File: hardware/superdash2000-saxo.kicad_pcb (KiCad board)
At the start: 2 copper layers, 77.5 x 59.7 mm, 21 parts, among them IC1 MAX4617CPE+, J1 Molex 34691-0161, U1 L7805, U2 TLV2372

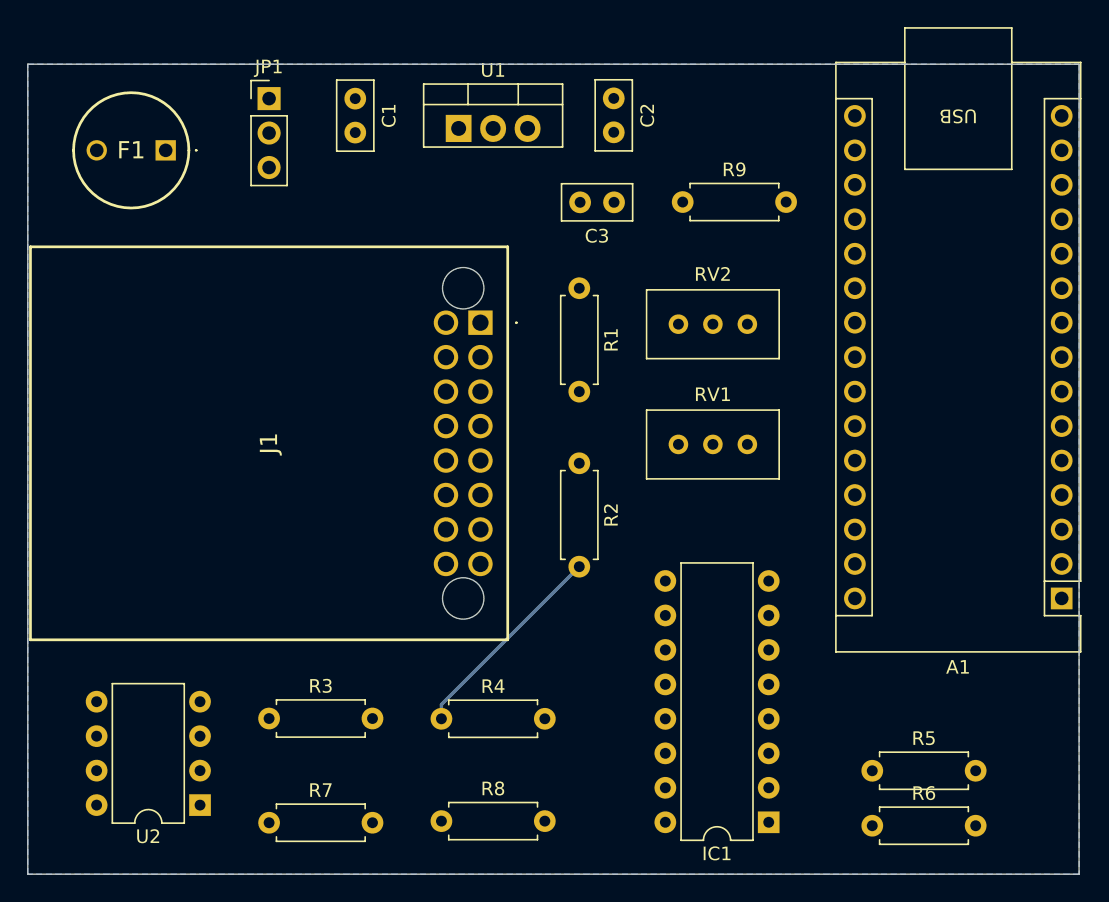
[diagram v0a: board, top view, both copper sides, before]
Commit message: hardware: Update pcb
Signed-off-by: Thomas Antonini <antonini.thomas@gmail.com>
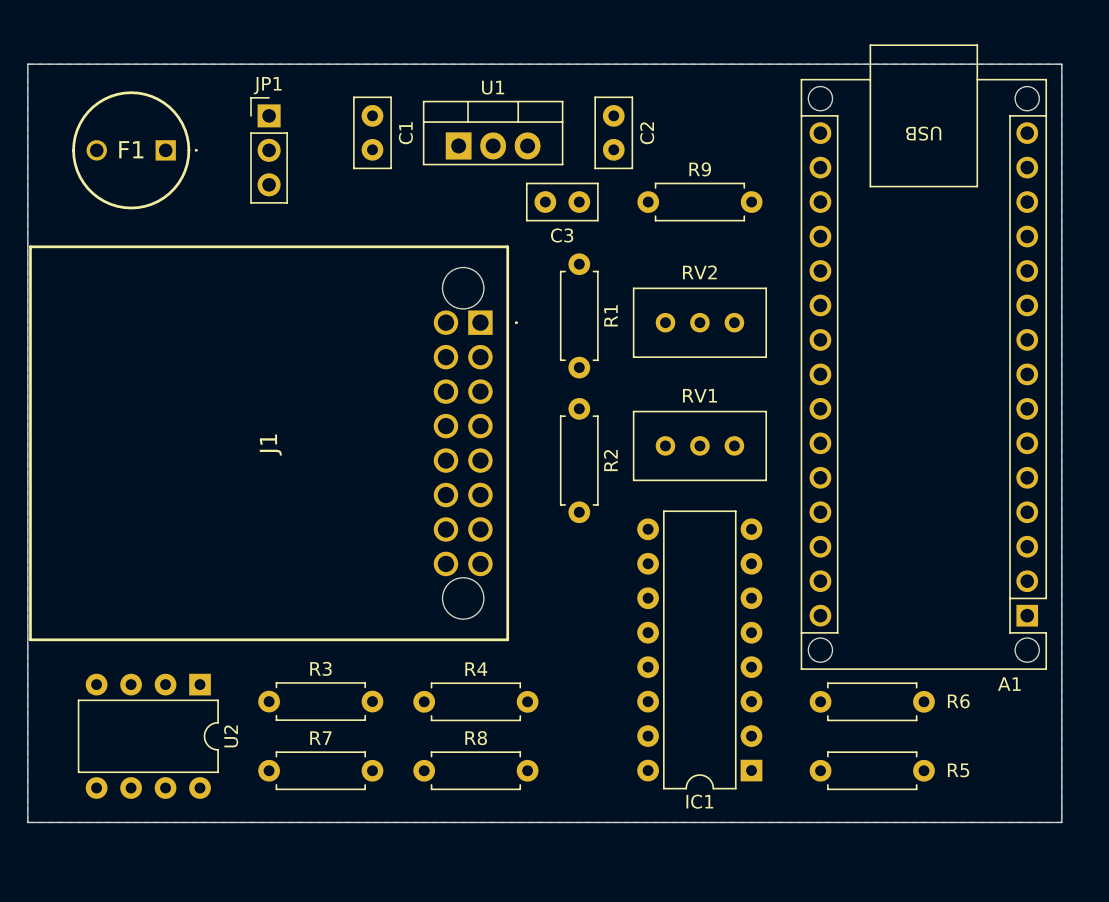
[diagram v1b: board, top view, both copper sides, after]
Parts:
- A1: footprint Module:Arduino_Nano -> Arduino_Nano_Every:Arduino_Nano_Every_WithMountingHoles
- moved R6 9.89 mm to (87.6, 101.6)
- moved U2 8.88 mm to (41.9, 100.3), turned to -90 degrees
- moved IC1 4.02 mm to (82.5, 106.7)
- moved R2 4.01 mm to (69.8, 80.0)
- moved R8 3.92 mm to (58.4, 106.7)
- moved R7 3.83 mm to (47.0, 106.7)
- moved R5 3.81 mm to (87.6, 106.7)
- moved A1 2.84 mm to (102.9, 95.2)
- moved C3 2.56 mm to (69.8, 64.8)
- moved R9 2.54 mm to (74.9, 64.8)
- moved C1 1.80 mm to (54.6, 58.4)
- moved R4 1.78 mm to (58.4, 101.6)
- moved R1 1.77 mm to (69.8, 69.3)
- moved C2 1.29 mm to (72.4, 58.4)
- moved U1 1.29 mm to (61.0, 60.6)
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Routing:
- net GND: track 15.4 -> 0.00 mm
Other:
- board size 77.5 x 59.7 mm -> 76.2 x 55.9 mm
